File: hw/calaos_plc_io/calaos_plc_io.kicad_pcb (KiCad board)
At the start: 2 copper layers, 41.7 x 90.4 mm, 167 parts, among them CON1 TerminalBlock, CON2 TerminalBlock, P1 SERIAL_DBG, P2 CONN_01X06, P4 CONN_01X04, Q1 Q_NPN_BCE, Q10 Q_NPN_BCE, Q11 Q_NPN_BCE, Q12 Q_NPN_BCE, Q13 Q_NPN_BCE, Q14 Q_NPN_BCE, Q15 Q_NPN_BCE, Q16 Q_NPN_BCE, Q2 Q_NPN_BCE, Q3 Q_NPN_BCE, Q4 Q_NPN_BCE, Q5 Q_NPN_BCE, Q6 Q_NPN_BCE, Q7 Q_NPN_BCE, Q8 Q_NPN_BCE, Q9 Q_NPN_BCE, U1 LM7824CT, U10 LTV-847, U11 LTV-847, U12 LTV-847, U13 LTV-847, U2 LM7805CT, U3 LD1117S33TR, U4 STM32F105R8, U5 MCP2551-I/SN, U6 LTV-847, U7 LTV-847, U8 LTV-847, U9 LTV-847, Y1 8MHz

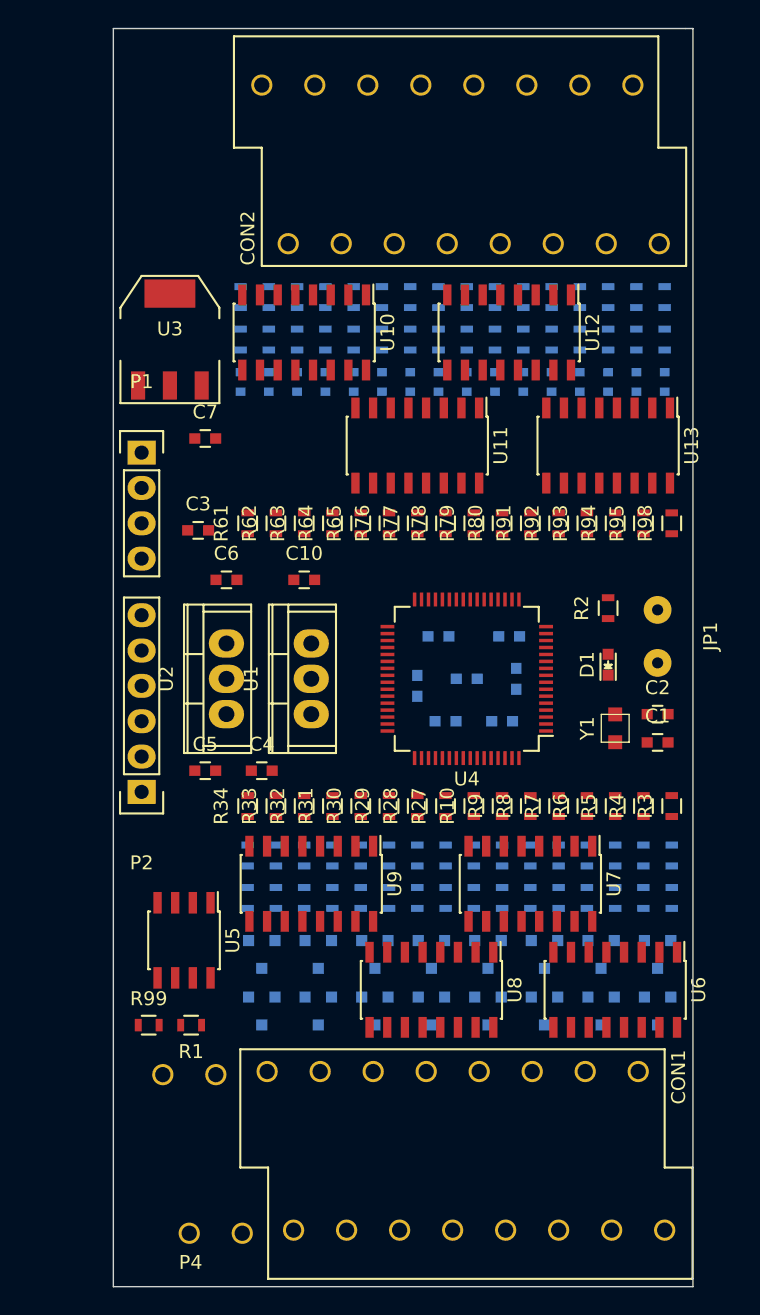
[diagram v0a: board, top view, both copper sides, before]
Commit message: Update schematics and pcb
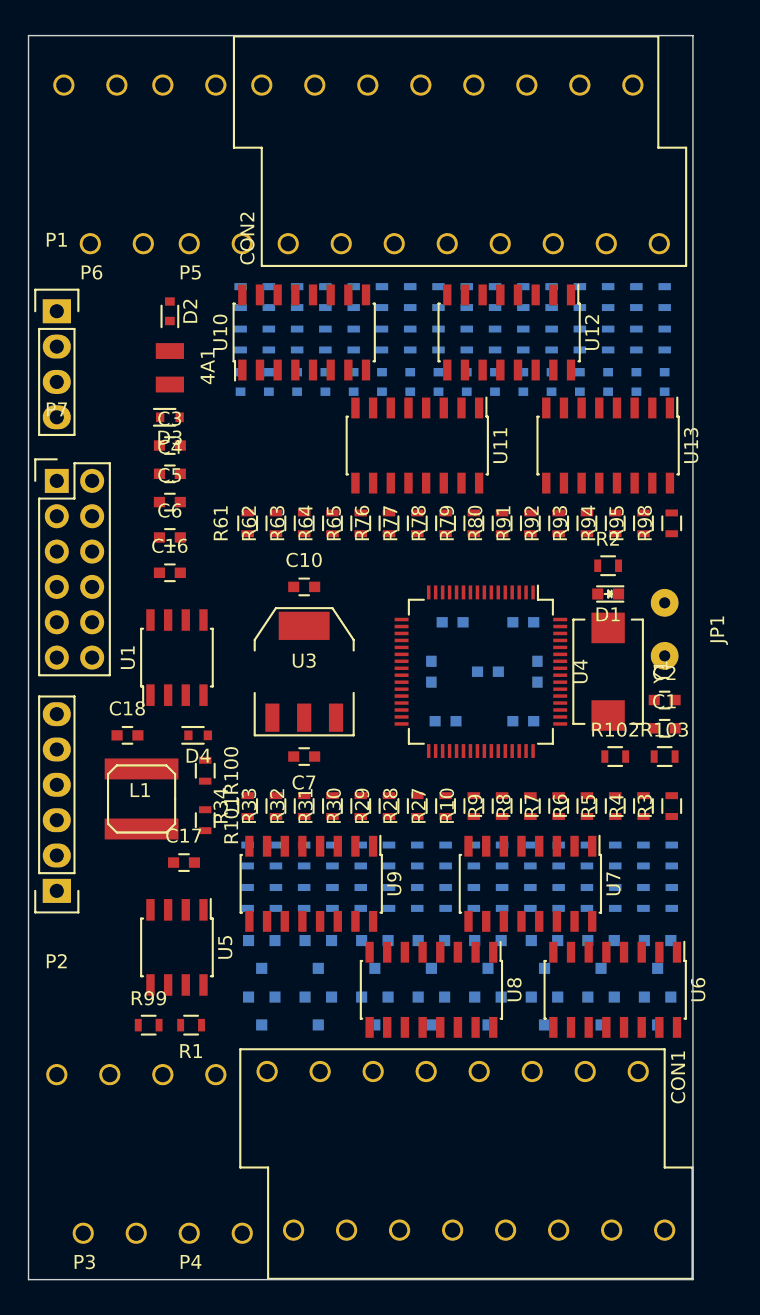
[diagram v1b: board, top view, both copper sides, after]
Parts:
- removed U2: LM7805CT, Power_Integrations:TO-220
- added 4A1: Fuse, Fuse_Holders_and_Fuses:Fuse_SMD1206_Reflow, F.Cu at (128.0, 71.6)
- added C16: 10uF, Capacitors_SMD:C_0603, F.Cu at (128.0, 86.4)
- added C17: 47uF, Capacitors_SMD:C_0603, F.Cu at (129.0, 107.2)
- added C18: 0.01uF, Capacitors_SMD:C_0603, F.Cu at (125.0, 98.0)
- added D2: D_Schottky, Diodes_SMD:SOD-523, F.Cu at (128.0, 67.6)
- added D3: TVS, Diodes_SMD:SOD-523, F.Cu at (128.0, 75.2)
- added D4: B340A-13-F, Diodes_SMD:SOD-523, F.Cu at (130.0, 98.0)
- added L1: 68uH, Inductors:SELF-WE-TPC_M, F.Cu at (126.0, 102.6)
- added P3: CONN_01X04, plc:Terminalbloc_1726040, F.Cu at (119.9, 122.4)
- added P5: CONN_01X04, plc:Terminalbloc_1726040, F.Cu at (127.5, 51.3)
- added P6: CONN_01X04, plc:Terminalbloc_1726040, F.Cu at (120.4, 51.3)
- added P7: CONN_02X06, Pin_Headers:Pin_Header_Straight_2x06, F.Cu at (119.9, 79.8)
- added R100: 10K, Resistors_SMD:R_0603, F.Cu at (130.6, 100.6)
- added R101: 3.24K, Resistors_SMD:R_0603, F.Cu at (130.6, 104.1)
- added R102: R, Resistors_SMD:R_0603, F.Cu at (160.0, 99.6)
- added R103: R, Resistors_SMD:R_0603, F.Cu at (163.6, 99.6)
- C3, C4: value 0.33uF -> 0.1uF
- C5, C6: value 0.1uF -> 10uF
- U1: value LM7824CT -> TPS5420D; footprint Power_Integrations:TO-220 -> Housings_SOIC:SOIC-8_3.9x4.9mm_Pitch1.27mm
- Y1: footprint Crystals_Oscillators_SMD:crystal_FA238-TSX3225 -> Crystals:Crystal_FOX-FE_SMD
- moved U3 25.8 mm to (137.7, 93.5)
- moved C7 23.9 mm to (137.7, 99.6), turned to 180 degrees
- moved C4 22.3 mm to (128.0, 79.2)
- moved C5 19.5 mm to (128.0, 81.3)
- moved P1 11.8 mm to (119.9, 67.6)
- moved U1 9.77 mm to (128.5, 92.5)
- moved P2 9.37 mm to (119.9, 109.2)
- moved C3 6.43 mm to (128.0, 77.2)
- moved C6 5.08 mm to (128.0, 83.8)
- moved D1 5.08 mm to (159.5, 87.9), turned to 180 degrees
- moved Y1 4.10 mm to (159.5, 93.5), turned to 270 degrees
- moved R2 3.05 mm to (159.5, 85.9), turned to 0 degrees
- moved C15 1.61 mm to (150.9, 93.5)
- moved C9 1.61 mm to (154.4, 93.5)
- moved C12 1.52 mm to (153.4, 97.0)
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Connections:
- C3 pad 1: VIN -> +24V
- C4 pad 1: VIN -> +24V
- C6 pad 1: +5V -> +24V
- R61 pad 2: /Inputs-1/I_0 -> /Inputs-1/I_1
- R62 pad 2: /Inputs-1/I_1 -> /Inputs-1/I_2
- R63 pad 2: /Inputs-1/I_2 -> /Inputs-1/I_3
- R64 pad 2: /Inputs-1/I_3 -> /Inputs-1/I_4
- R65 pad 2: /Inputs-1/I_4 -> /Inputs-1/I_5
- R76 pad 2: /Inputs-1/I_5 -> /Inputs-1/I_6
- R77 pad 2: /Inputs-1/I_6 -> /Inputs-1/I_7
- R78 pad 2: /Inputs-1/I_7 -> /Inputs-1/I_8
- R79 pad 2: /Inputs-1/I_8 -> /Inputs-1/I_9
- R80 pad 2: /Inputs-1/I_9 -> /Inputs-1/I_10
- R91 pad 2: /Inputs-1/I_10 -> /Inputs-1/I_11
- R92 pad 2: /Inputs-1/I_11 -> /Inputs-1/I_12
- R93 pad 2: /Inputs-1/I_12 -> /Inputs-1/I_13
- R94 pad 2: /Inputs-1/I_13 -> /Inputs-1/I_14
- R95 pad 2: /Inputs-1/I_14 -> /Inputs-1/I_15
- R98 pad 2: /Inputs-1/I_15 -> /Inputs-1/I_16
- U1 pad 1: VIN -> Net-(C18-Pad2)
- U1 pad 2: GND -> (no net)
- U1 pad 3: +24V -> (no net)
- U10 pad 10: /Inputs-1/I_3 -> /Inputs-1/I_4
- U10 pad 12: /Inputs-1/I_2 -> /Inputs-1/I_3
- U10 pad 14: /Inputs-1/I_1 -> /Inputs-1/I_2
- U10 pad 16: /Inputs-1/I_0 -> /Inputs-1/I_1
- U11 pad 10: /Inputs-1/I_7 -> /Inputs-1/I_8
- U11 pad 12: /Inputs-1/I_6 -> /Inputs-1/I_7
- U11 pad 14: /Inputs-1/I_5 -> /Inputs-1/I_6
- U11 pad 16: /Inputs-1/I_4 -> /Inputs-1/I_5
- U12 pad 10: /Inputs-1/I_11 -> /Inputs-1/I_12
- U12 pad 12: /Inputs-1/I_10 -> /Inputs-1/I_11
- U12 pad 14: /Inputs-1/I_9 -> /Inputs-1/I_10
- U12 pad 16: /Inputs-1/I_8 -> /Inputs-1/I_9
- U13 pad 10: /Inputs-1/I_15 -> /Inputs-1/I_16
- U13 pad 12: /Inputs-1/I_14 -> /Inputs-1/I_15
- U13 pad 14: /Inputs-1/I_13 -> /Inputs-1/I_14
- U13 pad 16: /Inputs-1/I_12 -> /Inputs-1/I_13
- U4 pad 14: (no net) -> PA0
- U4 pad 15: (no net) -> Net-(R102-Pad2)
- U4 pad 16: (no net) -> PA2
- U4 pad 17: (no net) -> PA3
- U4 pad 20: (no net) -> PA4
- U4 pad 21: (no net) -> PA5
- U4 pad 22: (no net) -> PA6
- U4 pad 23: (no net) -> PA7
- U4 pad 26: (no net) -> /Inputs-1/I_1
- U4 pad 27: (no net) -> /Inputs-1/I_2
- U4 pad 28: (no net) -> /Inputs-1/I_3
- U4 pad 29: (no net) -> /Inputs-1/I_11
- U4 pad 30: (no net) -> /Inputs-1/I_12
- U4 pad 33: (no net) -> /Inputs-1/I_13
- U4 pad 34: (no net) -> /Inputs-1/I_14
- U4 pad 35: (no net) -> /Inputs-1/I_15
- U4 pad 36: (no net) -> /Inputs-1/I_16
- U4 pad 41: (no net) -> PA8
- U4 pad 54: (no net) -> PD2
- U4 pad 55: (no net) -> /Inputs-1/I_4
- U4 pad 56: (no net) -> /Inputs-1/I_5
- U4 pad 57: (no net) -> /Inputs-1/I_6
- U4 pad 58: (no net) -> /Inputs-1/I_7
- U4 pad 59: (no net) -> /Inputs-1/I_8
- U4 pad 61: (no net) -> /Inputs-1/I_9
- U4 pad 62: (no net) -> /Inputs-1/I_10
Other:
- board size 41.7 x 90.4 mm -> 47.8 x 89.4 mm
